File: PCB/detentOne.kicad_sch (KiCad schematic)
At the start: 1 part, among them U3 ESP32-S3-WROOM-1(N16R8)

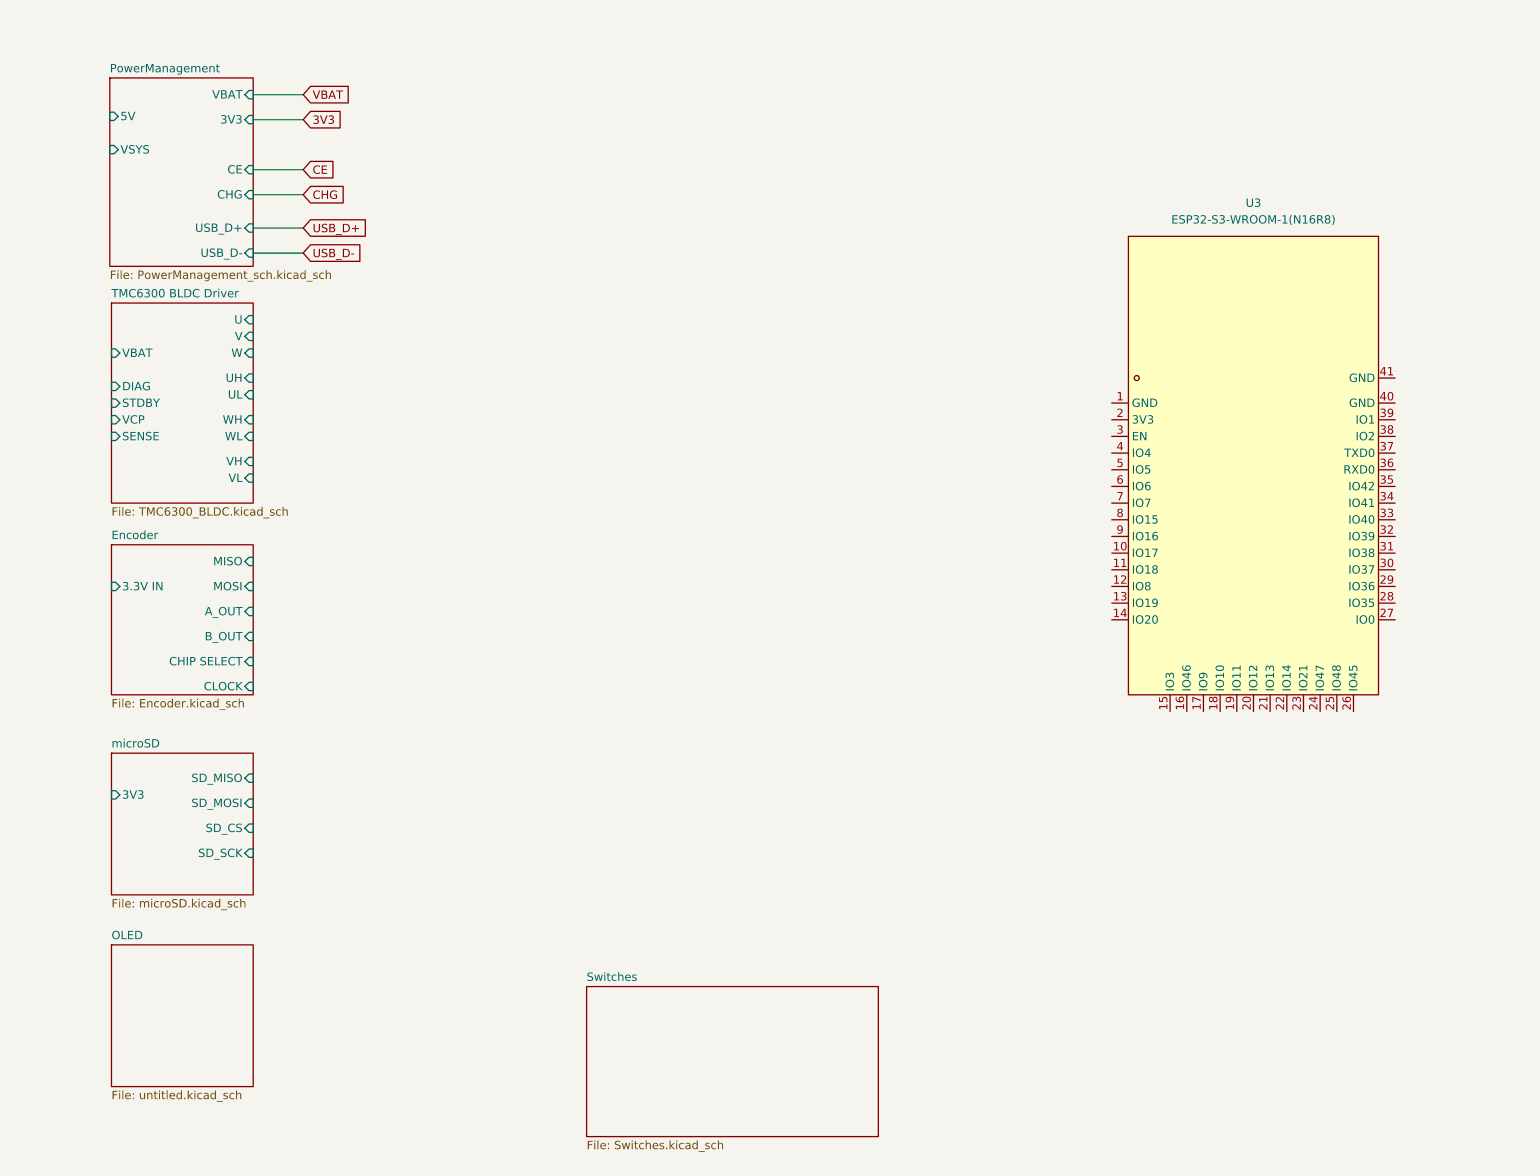
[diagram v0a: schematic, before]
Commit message: Finished schematic
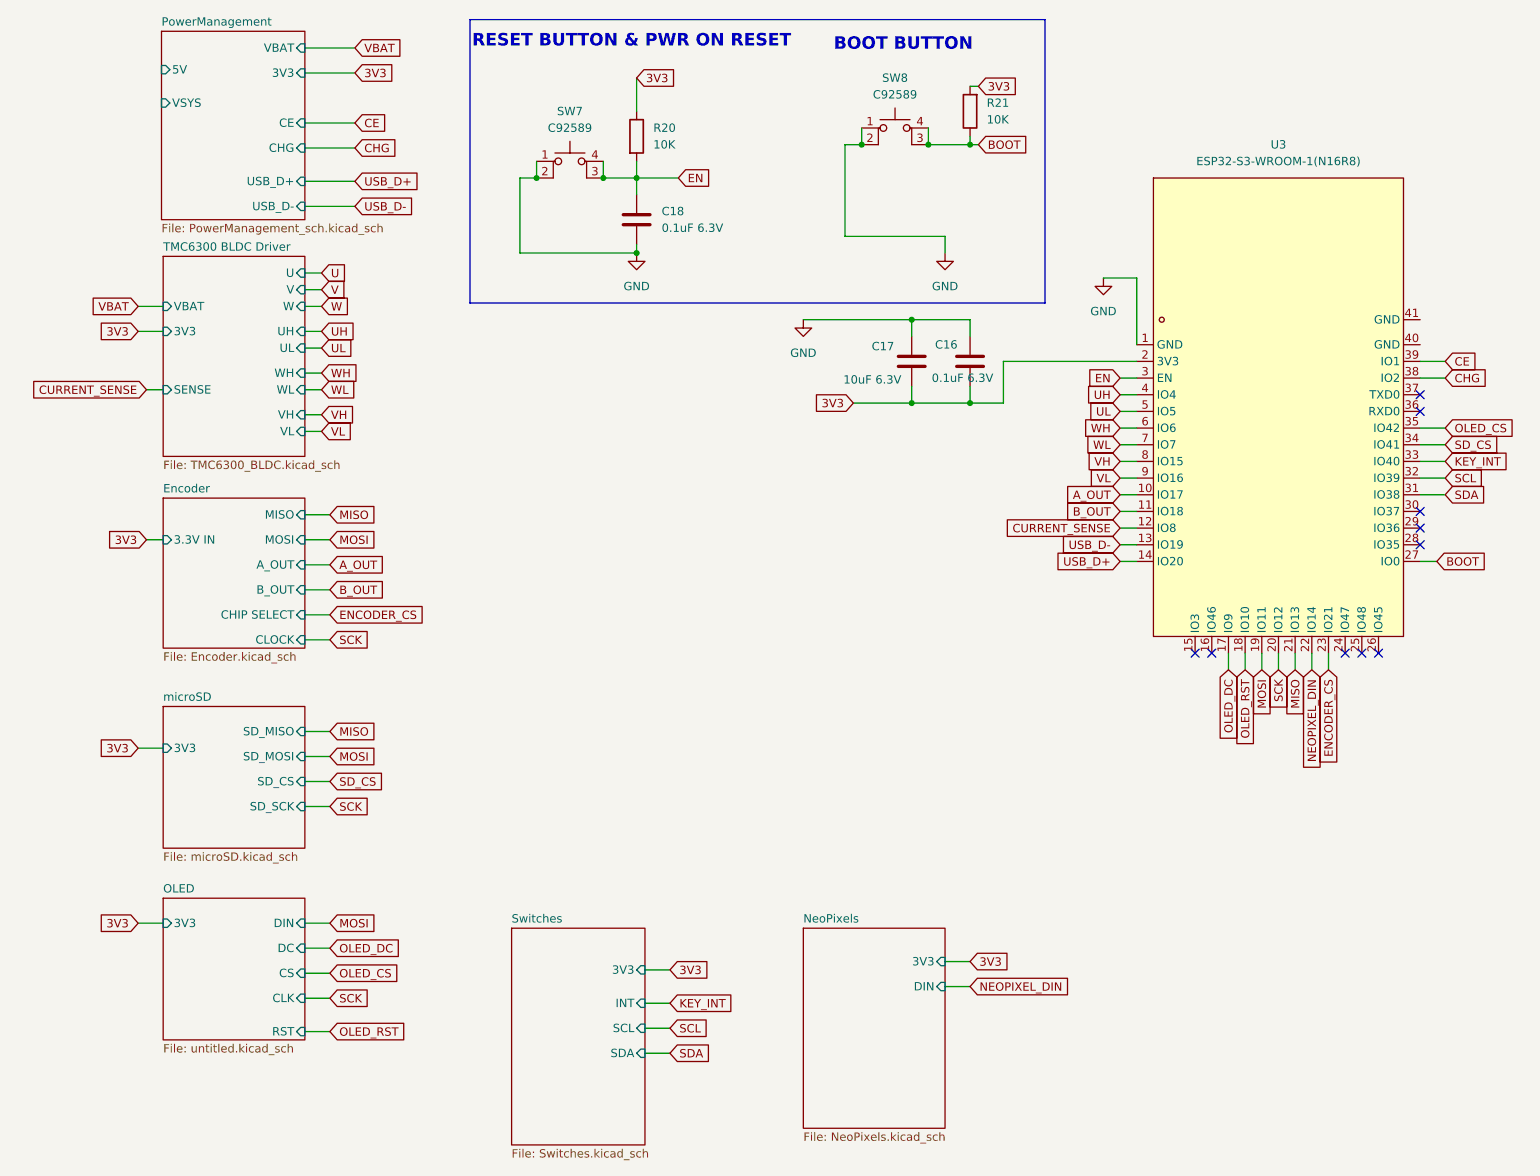
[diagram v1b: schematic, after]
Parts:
- added C16, C18: 0.1uF 6.3V, Capacitor_SMD:C_0603_1608Metric_Pad1.08x0.95mm_HandSolder, symbol Device:C
- added C17: 10uF 6.3V, Capacitor_SMD:C_0603_1608Metric_Pad1.08x0.95mm_HandSolder, symbol Device:C
- added R20, R21: 10K, Resistor_SMD:R_0603_1608Metric_Pad0.98x0.95mm_HandSolder, symbol Device:R
- added SW7, SW8: C92589, easyeda2kicad:KEY-SMD_4P-L4.2-W3.2-P2.20-LS5.1-TL, symbol Switch:SW_MEC_5E
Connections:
- net 3V3: now also U3.2 (3V3), C16.2, C17.2, R20.1, R21.2
- net CE: now also U3.39 (IO1)
- net CHG: now also U3.38 (IO2)
- net USB_D+: now also U3.14 (IO20)
- net USB_D-: now also U3.13 (IO19)
- net GND: now reaches U3.1 (GND)
- net GND: now also C16.1, C17.1, C18.2, SW7.1, SW7.2, SW8.1, SW8.2
- net A_OUT: now reaches U3.10 (IO17)
- net B_OUT: now reaches U3.11 (IO18)
- net CURRENT_SENSE: now reaches U3.12 (IO8)
- net OLED_DC: now reaches U3.17 (IO9)
- net OLED_RST: now reaches U3.18 (IO10)
- net MOSI: now reaches U3.19 (IO11)
- net SCK: now reaches U3.20 (IO12)
- net MISO: now reaches U3.21 (IO13)
- net NEOPIXEL_DIN: now reaches U3.22 (IO14)
- net ENCODER_CS: now reaches U3.23 (IO21)
- net BOOT: now reaches U3.27 (IO0)
- net BOOT: now also R21.1, SW8.3 (K), SW8.4 (A)
- net EN: now reaches U3.3 (EN)
- net EN: now also C18.1, R20.2, SW7.3 (K), SW7.4 (A)
- net SDA: now reaches U3.31 (IO38)
- net SCL: now reaches U3.32 (IO39)
- net KEY_INT: now reaches U3.33 (IO40)
- net SD_CS: now reaches U3.34 (IO41)
- net OLED_CS: now reaches U3.35 (IO42)
- net UH: now reaches U3.4 (IO4)
- net UL: now reaches U3.5 (IO5)
- net WH: now reaches U3.6 (IO6)
- net WL: now reaches U3.7 (IO7)
- net VH: now reaches U3.8 (IO15)
- net VL: now reaches U3.9 (IO16)
- no-connect marks 0 -> 10
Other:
- added sheet NeoPixels (NeoPixels.kicad_sch)
- sheet OLED ports: added 3V3, CLK, CS, DC, DIN, RST; removed none
- sheet Switches ports: added 3V3, INT, SCL, SDA; removed none
- sheet TMC6300 BLDC Driver ports: added 3V3; removed DIAG, STDBY, VCP
- note added: "BOOT BUTTON"
- note added: "RESET BUTTON & PWR ON RESET"
- moved on the sheet: U3

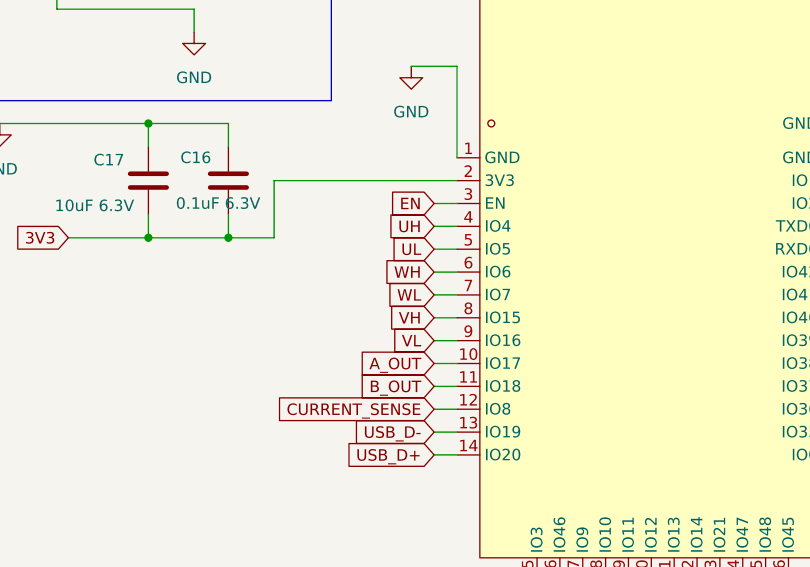
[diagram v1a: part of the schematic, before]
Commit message: PCB layout done
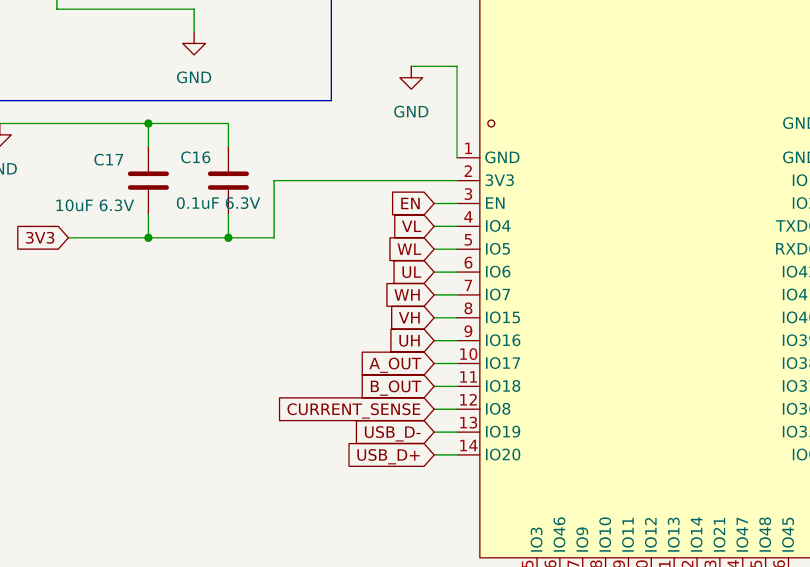
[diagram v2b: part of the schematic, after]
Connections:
- net UH: now also U3.9 (IO16); no longer U3.4 (IO4)
- net UL: now also U3.6 (IO6); no longer U3.5 (IO5)
- net VL: now also U3.4 (IO4); no longer U3.9 (IO16)
- net WH: now also U3.7 (IO7); no longer U3.6 (IO6)
- net WL: now also U3.5 (IO5); no longer U3.7 (IO7)
